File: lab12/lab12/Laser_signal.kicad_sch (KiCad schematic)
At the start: 48 parts, among them U1 MC7805CT-BP, U10 LM324, U14 LM324, U2 NE555D, U5 LM324, U8 LM339

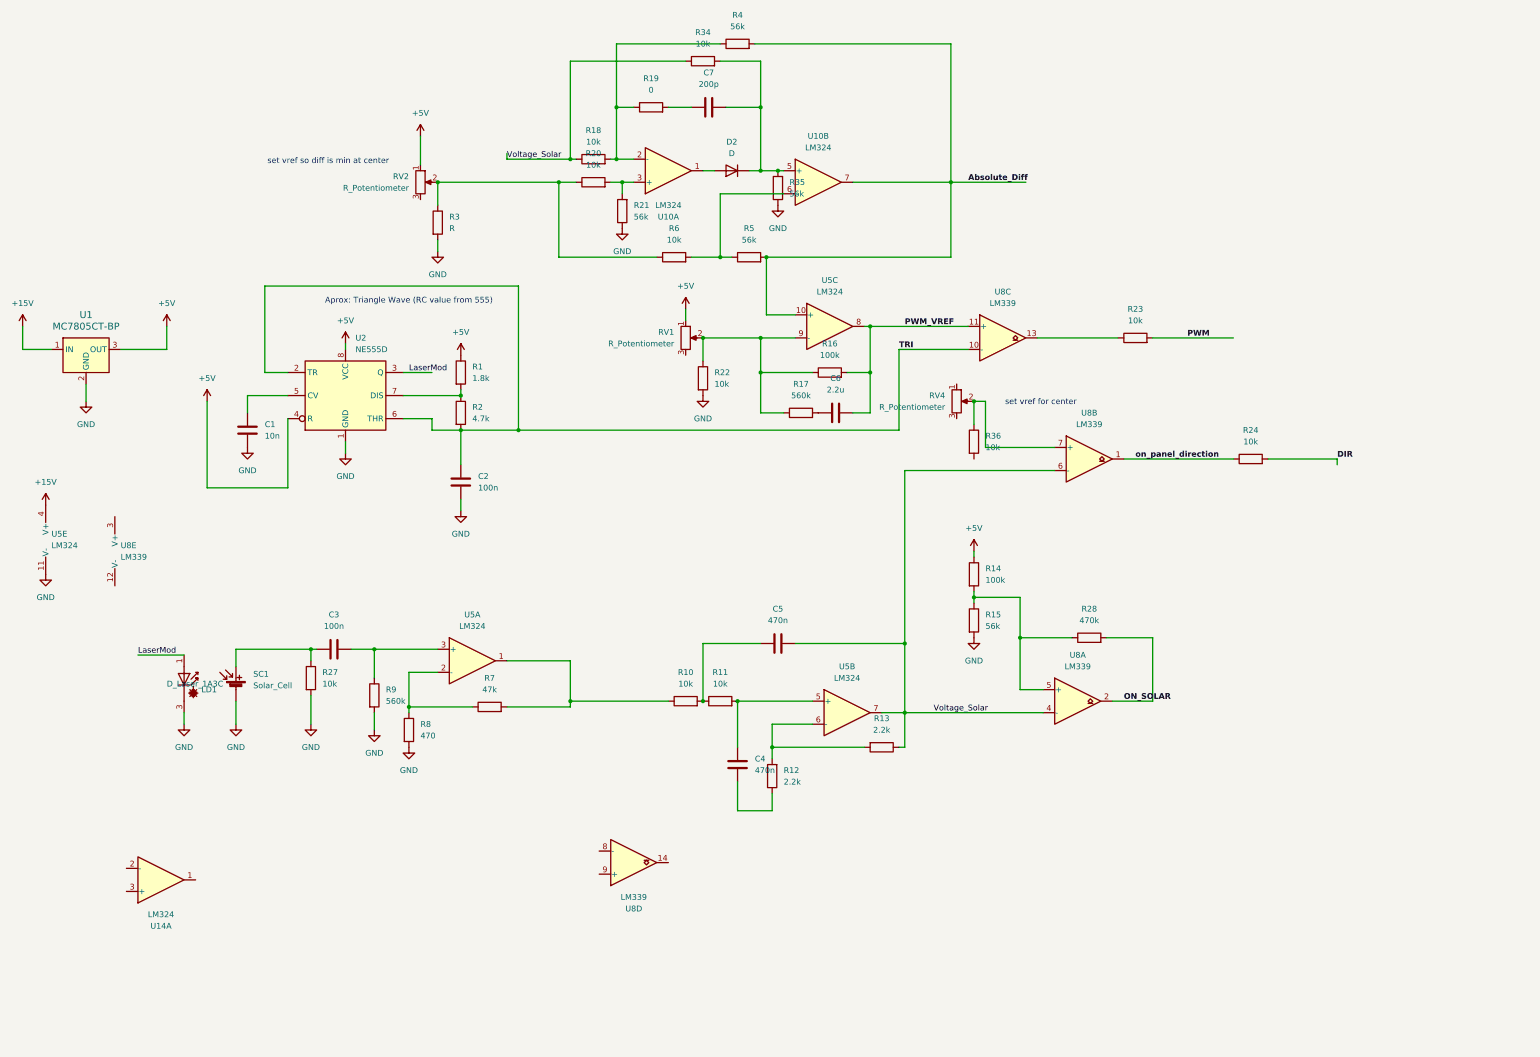
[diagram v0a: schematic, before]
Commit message: Code for lab 13
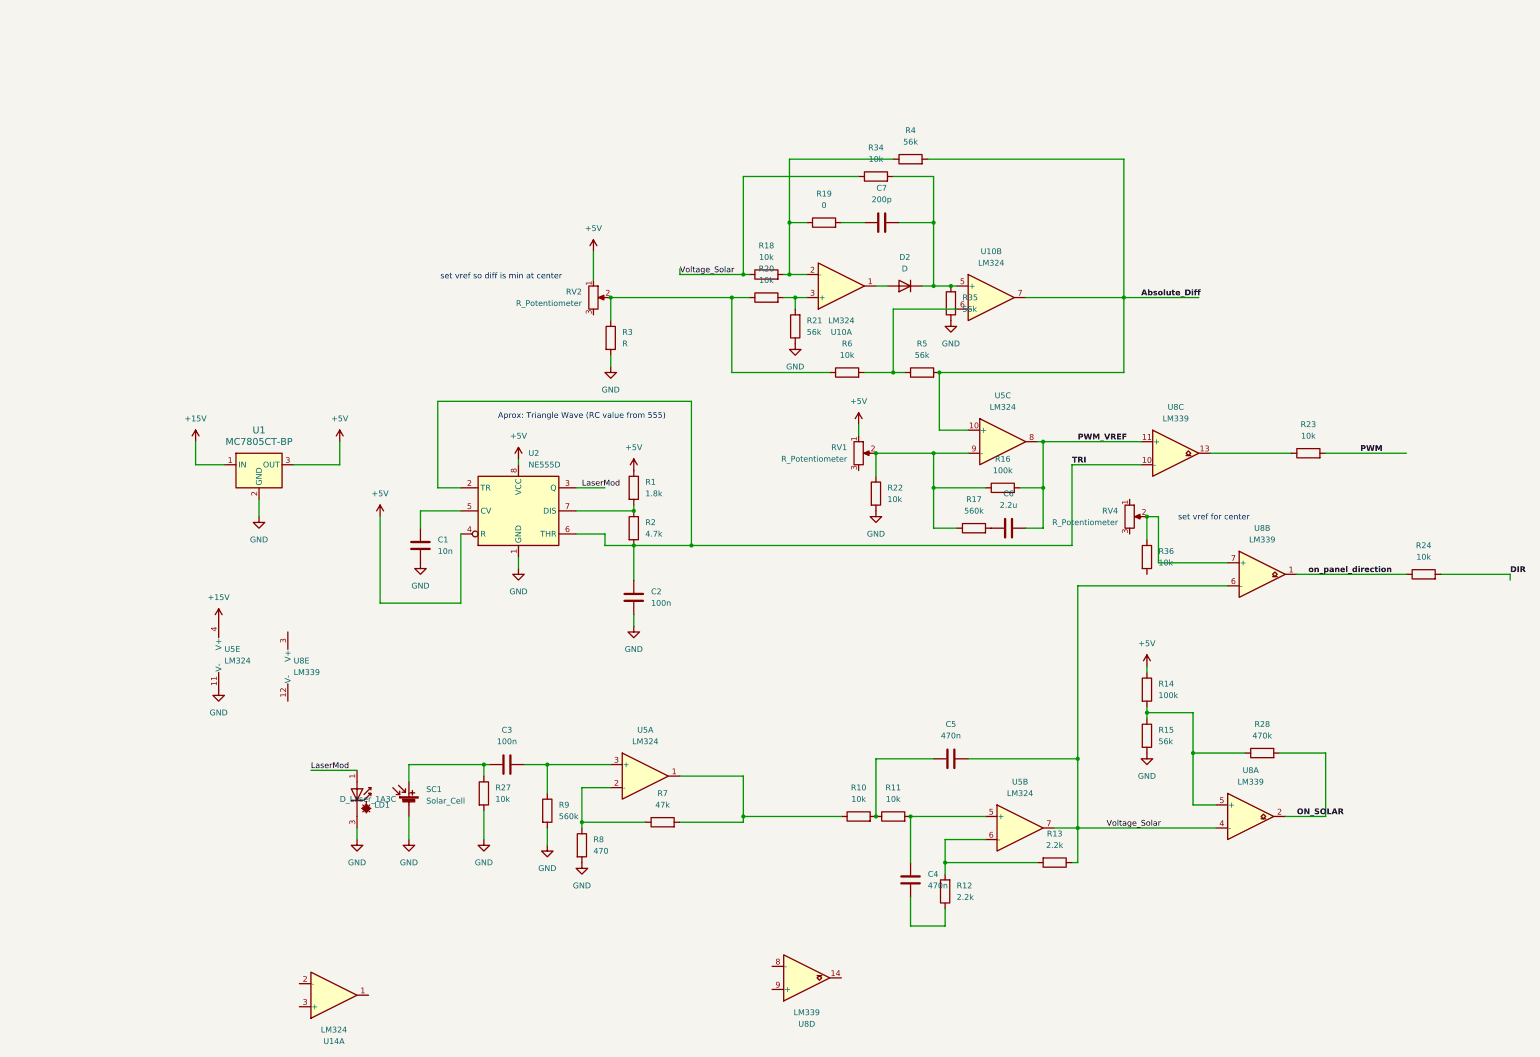
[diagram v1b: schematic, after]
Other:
- company: (none) -> CWRU
- moved on the sheet: C1, C2, C3, C4, C5, C6, C7, D2, LD1, R1, R10, R11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
